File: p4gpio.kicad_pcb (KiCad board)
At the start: 4 copper layers, 88.9 x 23 mm, 93 parts, among them J1 C2760486, J10 Conn_01x04_Socket, J11 Conn_01x04, J2 C2760486, J3 Conn_01x08_Pin, J4 Conn_01x08_Pin, J5 Conn_01x08_Pin, J6 Conn_01x08_Pin, J7 Conn_01x08_Pin, J8 Conn_01x08_Pin, J9 Conn_01x04_Socket, Q1 MBT3906DW1, Q2 AO3401A, Q3 MBT3906DW1, Q4 AO3401A, U1 TLV62569DBV, U3 W25Q128JVS, U4 TLV62569DBV, Y1 40MHz(+-10 ppm) C501798

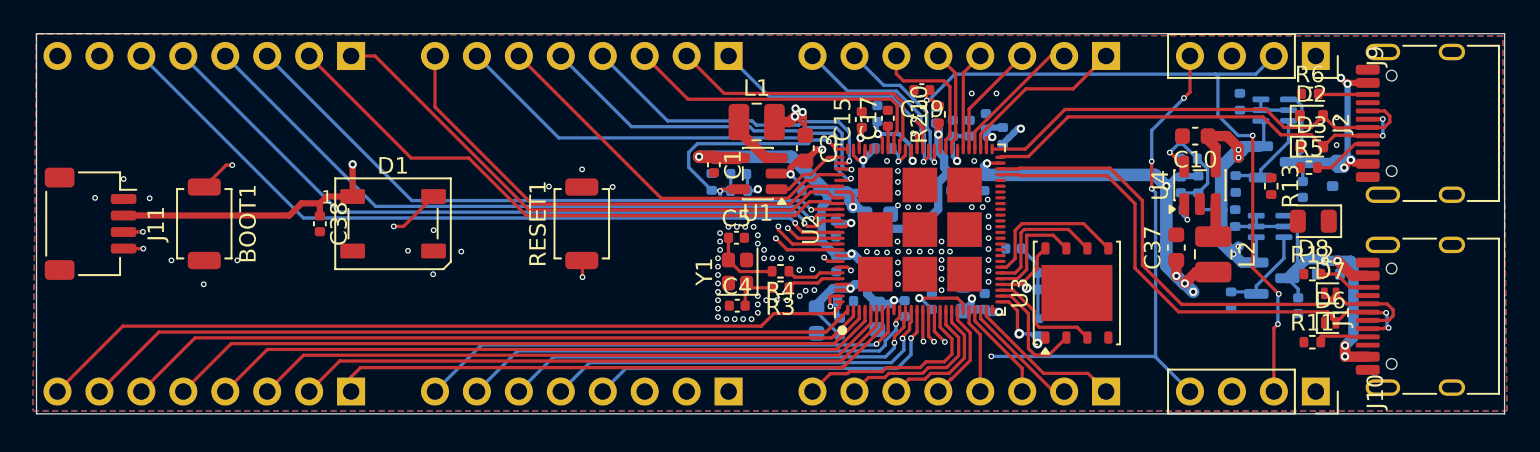
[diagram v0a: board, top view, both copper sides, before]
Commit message: Done?
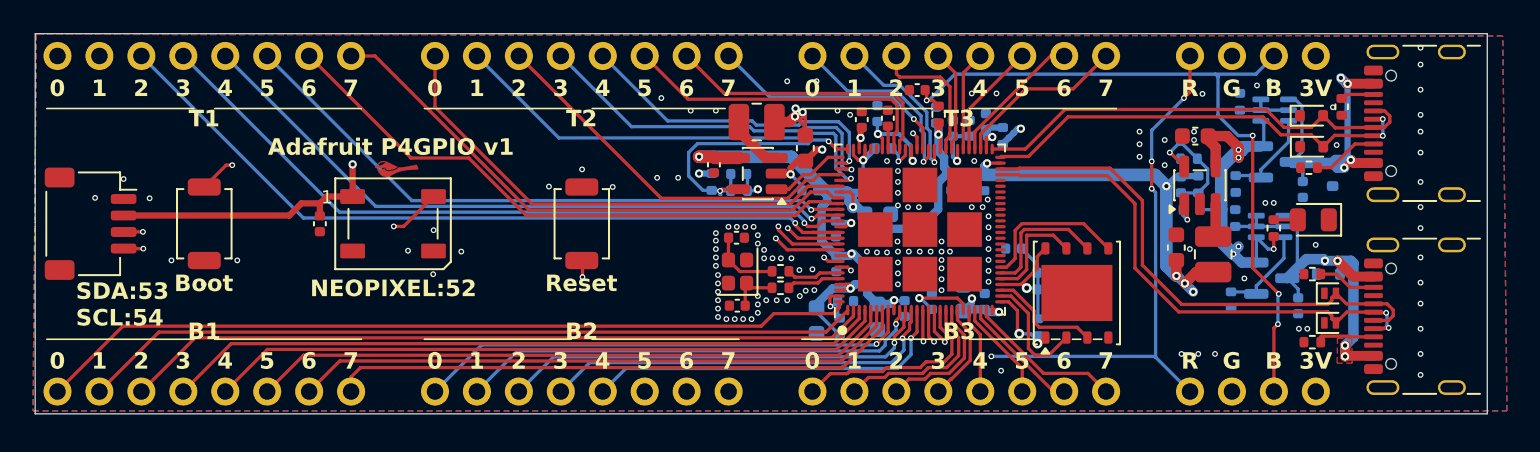
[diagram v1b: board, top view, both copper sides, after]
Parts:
- added G***: LOGO, chickadee:chickadee_1mm_fcu, F.Cu at (144.5, 81.0)
- J1, J2: footprint Connector_USB:USB_C_Receptacle_HRO_TYPE-C-31-M-12 -> Adafruit:USB_C_Receptacle_HRO_TYPE-C-31-M-31
- moved R13 2.54 mm to (197.6, 84.6), turned to 90 degrees
- moved R6 2.08 mm to (201.7, 77.2), turned to 90 degrees
- moved C39 0.28 mm to (176.0, 76.2)
- moved D8 0.09 mm to (200.0, 84.1)
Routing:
- net /HS_VBUS: track 20.1 -> 22.4 mm
- net VBUS: track 27.9 -> 30.0 mm, vias 4 -> 5
- net /FS_VBUS: track 18.4 -> 19.8 mm
- net Net-(D8-A): track 0.00 -> 1.46 mm
- net Net-(J2-CC1): track 2.87 -> 3.99 mm
- net Net-(J2-CC2): track 3.01 -> 2.02 mm
- net GND: track 4.88 -> 5.65 mm, vias 92 -> 138
- added copper zone on F.Cu, net /HS_VBUS
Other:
- board size 88.9 x 23 mm -> 87.9 x 23 mm
- board text added: "0"
- board text added: "1"
- board text added: "2"
- board text added: "3"
- board text added: "3V"
- board text added: "4"
- board text added: "5"
- board text added: "6"
- board text added: "7"
- board text added: "Adafruit P4GPIO v1"
- board text added: "B"
- board text added: "B1"
- board text added: "B2"
- board text added: "B3"
- board text added: "Boot"
- board text added: "G"
- board text added: "NEOPIXEL:52"
- board text added: "R"
- board text added: "Reset"
- board text added: "SDA:53 SCL:54"
- board text added: "T1"
- board text added: "T2"
- board text added: "T3"
